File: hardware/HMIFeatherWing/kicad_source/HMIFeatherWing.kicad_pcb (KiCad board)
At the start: 2 copper layers, 72 x 30 mm, 25 parts, among them CN1 ARDUINO_MKR, Q1 2N7002, SW1 ALPS_SKRH, SW6 TAST_VER

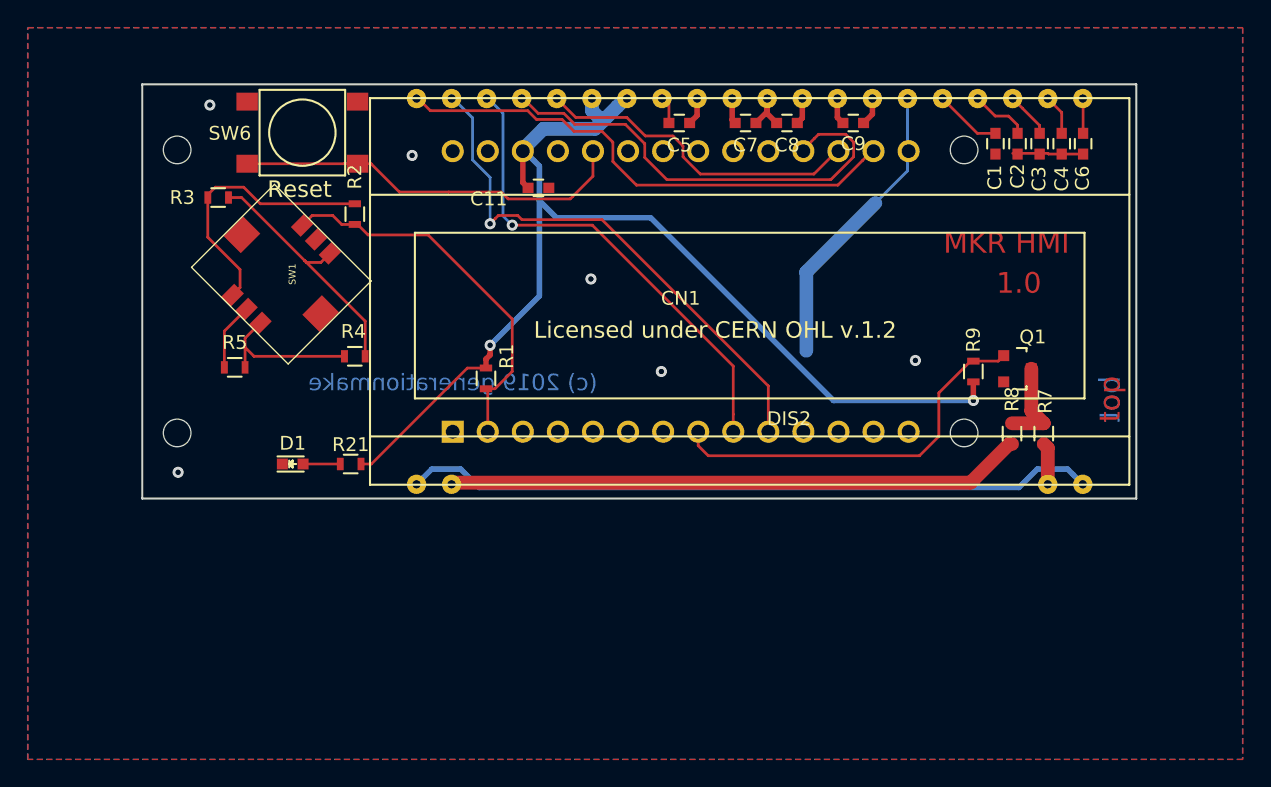
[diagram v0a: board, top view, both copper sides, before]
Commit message: made schematic and layout
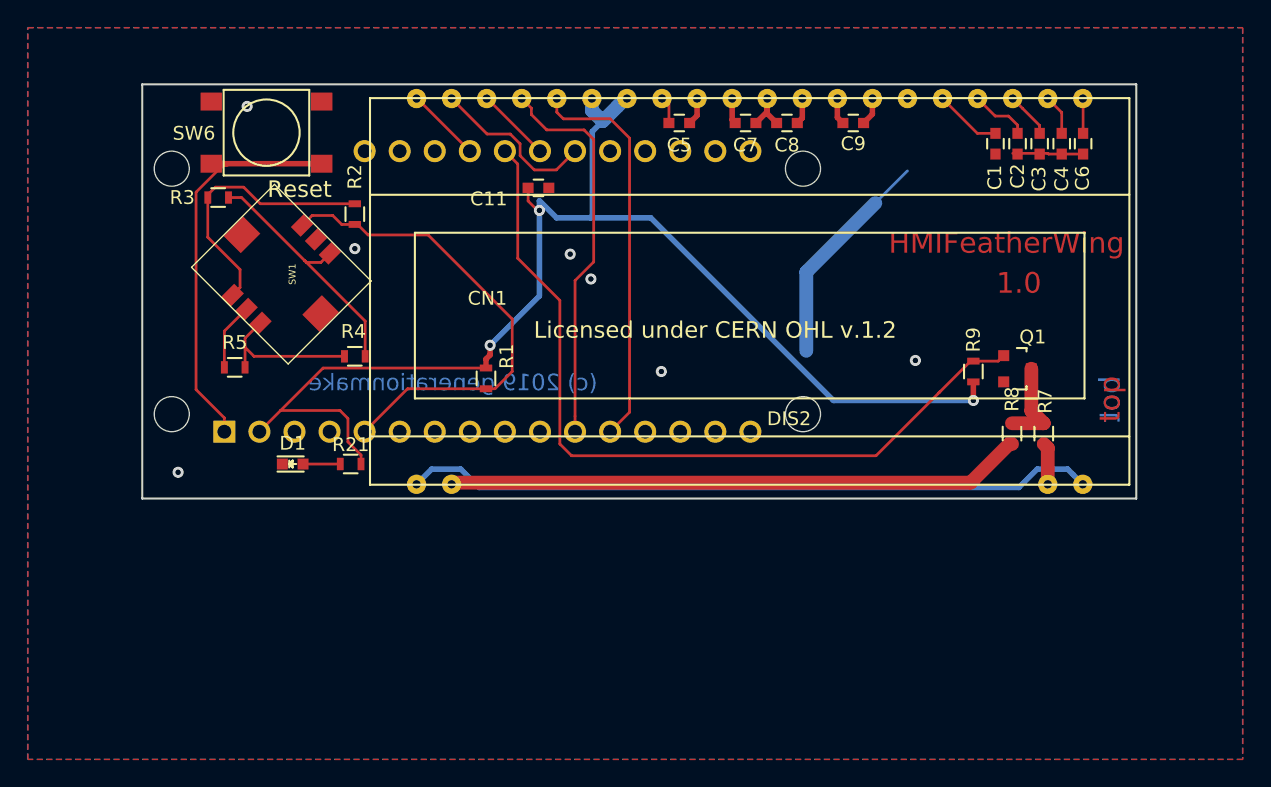
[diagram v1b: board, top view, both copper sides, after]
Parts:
- CN1: value ARDUINO_MKR -> ADAFRUIT_FEATHER; footprint MODULE_compute:ARDUINO_MKR_HOLES -> MODULE_compute:ADAFRUIT_FEATHER_HOLES
- moved CN1 14.0 mm to (76.0, 96.0)
- moved SW6 2.60 mm to (60.0, 84.5)
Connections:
- CN1 pad 1: Net-(CN1-Pad1) -> /RESET
- CN1 pad 10: /DIS_RESET -> (no net)
- CN1 pad 11: Net-(CN1-Pad11) -> /DIS_CLK
- CN1 pad 12: Net-(CN1-Pad12) -> /DIS_SI
- CN1 pad 16: /DIS_CS -> GND
- CN1 pad 17: /DIS_SI -> (no net)
- CN1 pad 18: /DIS_CLK -> (no net)
- CN1 pad 2: /KEYPAD_A0 -> +3V3
- CN1 pad 22: Net-(CN1-Pad22) -> /DIS_RESET
- CN1 pad 23: Net-(CN1-Pad23) -> /DIS_A0
- CN1 pad 24: /RESET -> /DISPLAY_BL
- CN1 pad 25: GND -> /DIS_CS
- CN1 pad 26: +3V3 -> (no net)
- CN1 pad 4: Net-(CN1-Pad4) -> GND
- CN1 pad 5: Net-(CN1-Pad5) -> /KEYPAD_A0
- CN1 pad 8: /DISPLAY_BL -> (no net)
- CN1 pad 9: /DIS_A0 -> (no net)
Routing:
- net /DIS_CS: track 37.6 -> 5.44 mm
- net /DISPLAY_BL: track 28.4 -> 58.5 mm
- net /DIS_A0: track 34.9 -> 5.44 mm, vias 1 -> 0
- net /DIS_RESET: track 39.0 -> 12.1 mm, vias 1 -> 0
- net +3V3: track 82.8 -> 93.6 mm, vias 2 -> 3
- net /KEYPAD_A0: track 27.9 -> 35.1 mm
- net GND: track 28.6 -> 23.3 mm, vias 6 -> 7
- net /DIS_SI: track 23.9 -> 28.9 mm
- net /DIS_CLK: track 33.2 -> 28.4 mm
- net /RESET: track 28.6 -> 30.5 mm
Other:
- board text added: "HMIFeatherWing"
- board text removed: "MKR HMI"
